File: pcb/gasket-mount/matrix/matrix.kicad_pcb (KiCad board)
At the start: 2 copper layers, 228.6 x 76.2 mm, 104 parts

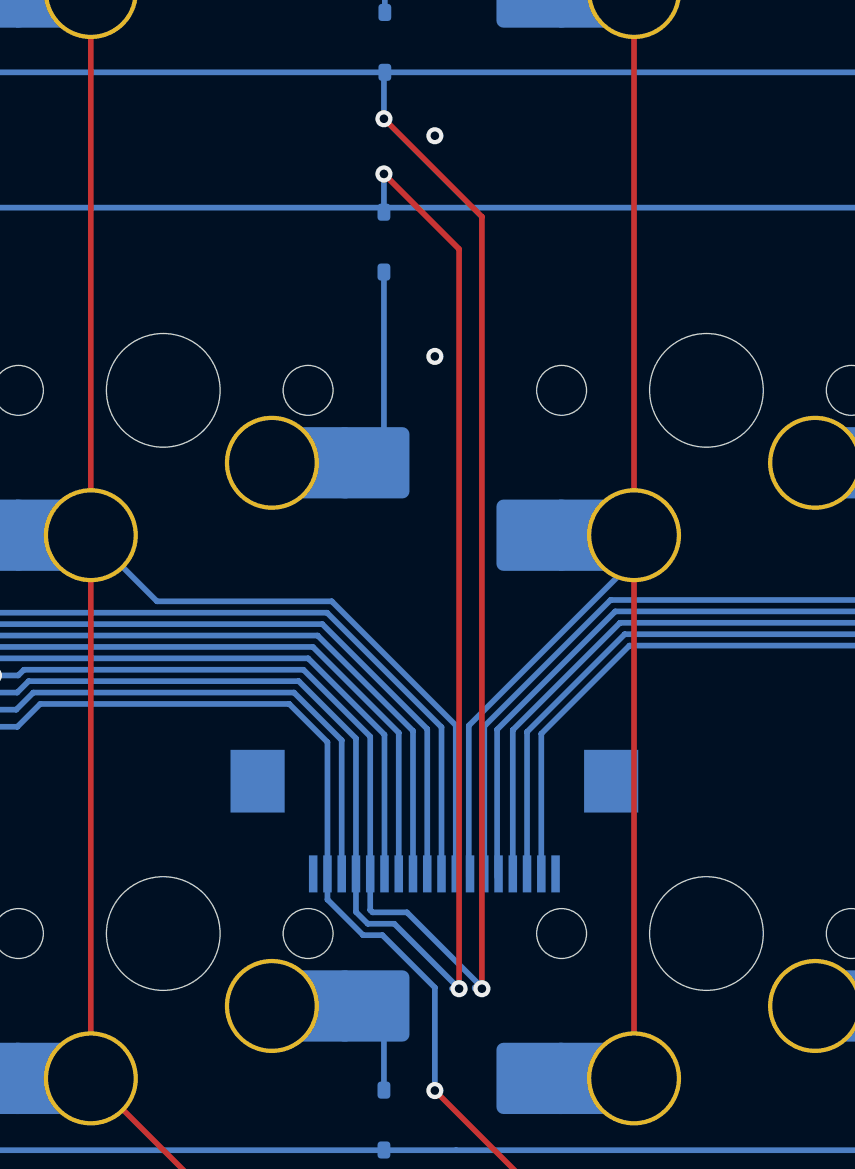
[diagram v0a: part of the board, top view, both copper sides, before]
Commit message: I finally ordered\!
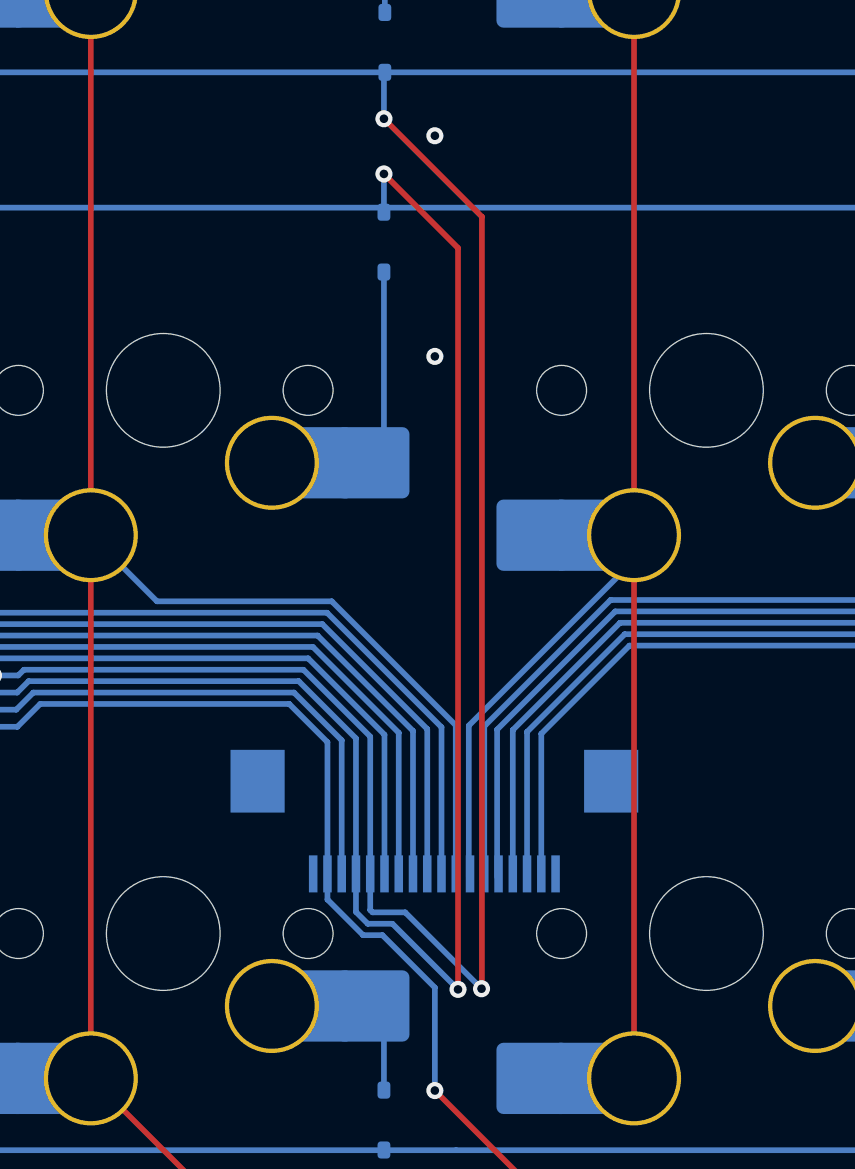
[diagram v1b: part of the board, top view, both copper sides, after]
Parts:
- U1: value ~ -> TF31-18S-0.5SH(800)
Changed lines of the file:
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@@
 			)
 		)
-		(property "Value" "~"
+		(property "Value" "TF31-18S-0.5SH(800)"
 			(at 0 -4.7455 0)
 			(layer "B.Fab")
@@
 	)
 	(segment
+		(start 151.668627 109.090924)
+		(end 151.655892 109.090924)
+		(width 0.2)
+		(layer "F.Cu")
+		(net "ROW1")
+	)
+	(segment
 		(start 148.232688 78.581184)
 		(end 151.668627 82.017123)
@@
 	)
 	(segment
+		(start 151.655892 109.090924)
+		(end 151.655792 109.091024)
+		(width 0.2)
+		(layer "F.Cu")
+		(net "ROW1")
+	)
+	(segment
 		(start 131.415124 80.813604)
 		(end 131.415124 96.023686)
@@
 	)
 	(via
-		(at 151.668627 109.090924)
+		(at 151.655792 109.091024)
 		(size 0.6)
 		(drill 0.3)
@@
 	)
 	(segment
-		(start 149.03964 106.413411)
-		(end 151.668627 109.042398)
+		(start 151.655792 109.091024)
+		(end 148.978179 106.413411)
 		(width 0.2)
 		(layer "B.Cu")
@@
 	)
 	(segment
-		(start 151.418627 109.042398)
-		(end 151.418627 109.090924)
-		(width 0.2)
-		(layer "B.Cu")
-		(net "ROW1")
-	)
-	(segment
 		(start 147.752224 106.332698)
 		(end 147.832937 106.413411)
@@
 	)
 	(segment
-		(start 149.03964 106.413411)
+		(start 148.978179 106.413411)
 		(end 147.832937 106.413411)
 		(width 0.2)
@@
 	)
 	(segment
-		(start 130.96864 96.142888)
-		(end 133.530585 98.704833)
+		(start 150.831475 109.115237)
+		(end 150.831475 83.114735)
 		(width 0.2)
 		(layer "F.Cu")
@@
 	)
 	(segment
-		(start 133.530585 98.704833)
-		(end 133.884322 98.704833)
+		(start 148.232688 80.515948)
+		(end 150.831475 83.114735)
 		(width 0.2)
 		(layer "F.Cu")
@@
 	)
 	(segment
-		(start 129.182704 80.36712)
-		(end 130.96864 82.153056)
+		(start 130.96864 96.142888)
+		(end 133.530585 98.704833)
 		(width 0.2)
 		(layer "F.Cu")
@@
 	)
 	(segment
-		(start 150.868624 109.090924)
-		(end 150.868624 83.151884)
+		(start 133.530585 98.704833)
+		(end 133.884322 98.704833)
 		(width 0.2)
 		(layer "F.Cu")
@@
 	)
 	(segment
-		(start 130.96864 82.153056)
-		(end 130.96864 96.142888)
+		(start 129.182704 80.36712)
+		(end 130.96864 82.153056)
 		(width 0.2)
 		(layer "F.Cu")
@@
 	)
 	(segment
-		(start 148.232688 80.515948)
-		(end 150.868624 83.151884)
+		(start 130.96864 82.153056)
+		(end 130.96864 96.142888)
 		(width 0.2)
 		(layer "F.Cu")
@@
 	)
 	(via
-		(at 148.232688 80.515948)
+		(at 150.831475 109.115237)
 		(size 0.6)
 		(drill 0.3)
@@
 	)
 	(via
-		(at 150.868624 109.090924)
+		(at 148.232688 80.515948)
 		(size 0.6)
 		(drill 0.3)
@@
 	)
 	(segment
+		(start 150.831475 109.114482)
+		(end 148.530404 106.813411)
+		(width 0.2)
+		(layer "B.Cu")
+		(net "ROW2")
+	)
+	(segment
 		(start 135.771984 98.304833)
 		(end 145.244207 98.304833)
@@
 	)
 	(segment
-		(start 148.596341 106.813411)
-		(end 150.868624 109.085695)
-		(width 0.2)
-		(layer "B.Cu")
-		(net "ROW2")
-	)
-	(segment
-		(start 147.667251 106.813411)
-		(end 148.596341 106.813411)
-		(width 0.2)
-		(layer "B.Cu")
-		(net "ROW2")
-	)
-	(segment
 		(start 52.982857 81.698506)
 		(end 262.532857 81.698507)
@@
 	)
 	(segment
-		(start 150.618624 109.085695)
-		(end 150.618624 109.090924)
-		(width 0.2)
-		(layer "B.Cu")
-		(net "ROW2")
-	)
-	(segment
 		(start 148.232733 81.857257)
 		(end 148.232733 80.515993)
@@
 	)
 	(segment
+		(start 150.831475 109.115237)
+		(end 150.831475 109.114482)
+		(width 0.2)
+		(layer "B.Cu")
+		(net "ROW2")
+	)
+	(segment
 		(start 129.182857 81.698507)
 		(end 129.182857 80.367273)
@@
 		(width 0.2)
 		(layer "B.Cu")
+		(net "ROW2")
+	)
+	(segment
+		(start 147.667251 106.813411)
+		(end 148.530404 106.813411)
+		(width 0.2)
+		(layer "B.Cu")
